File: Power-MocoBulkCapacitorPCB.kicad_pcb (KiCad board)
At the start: 2 copper layers, 120.5 x 44 mm, 142 parts, among them J1 Conn_01x02

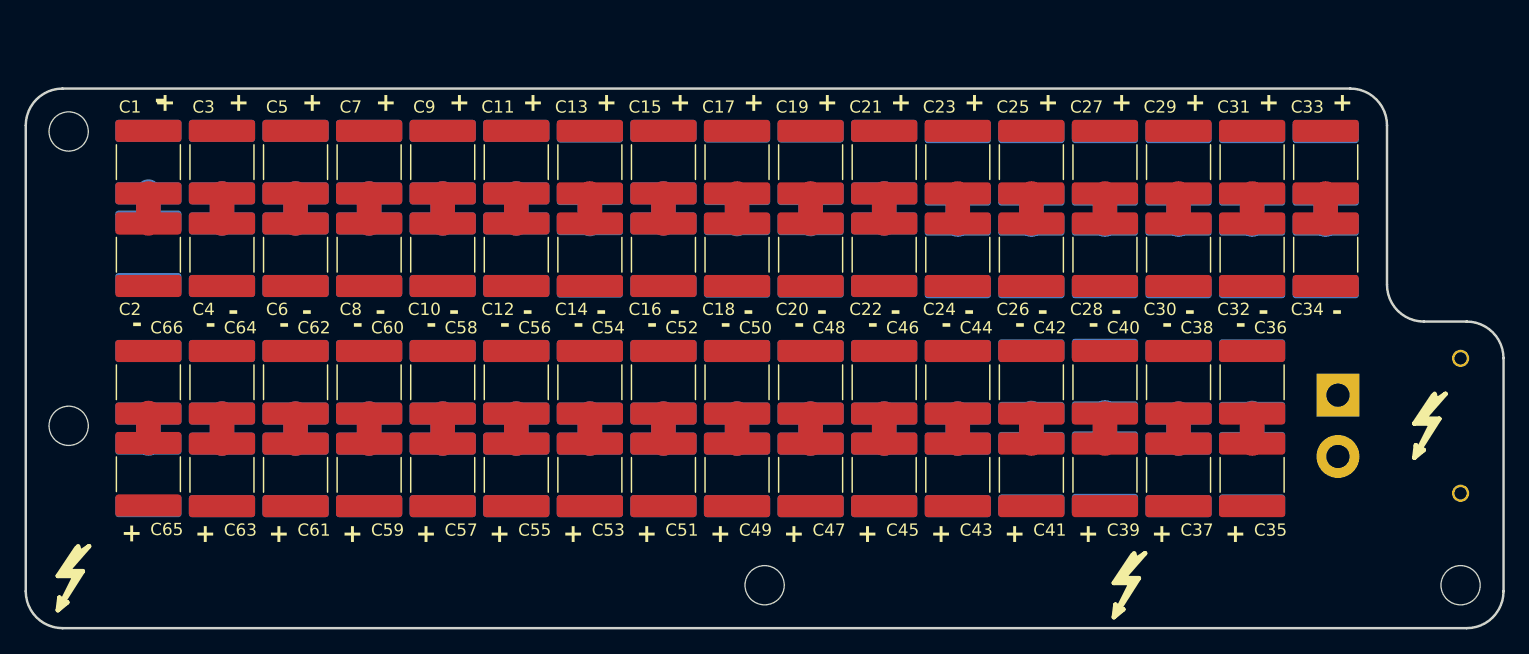
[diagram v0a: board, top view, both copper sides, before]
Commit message: holes
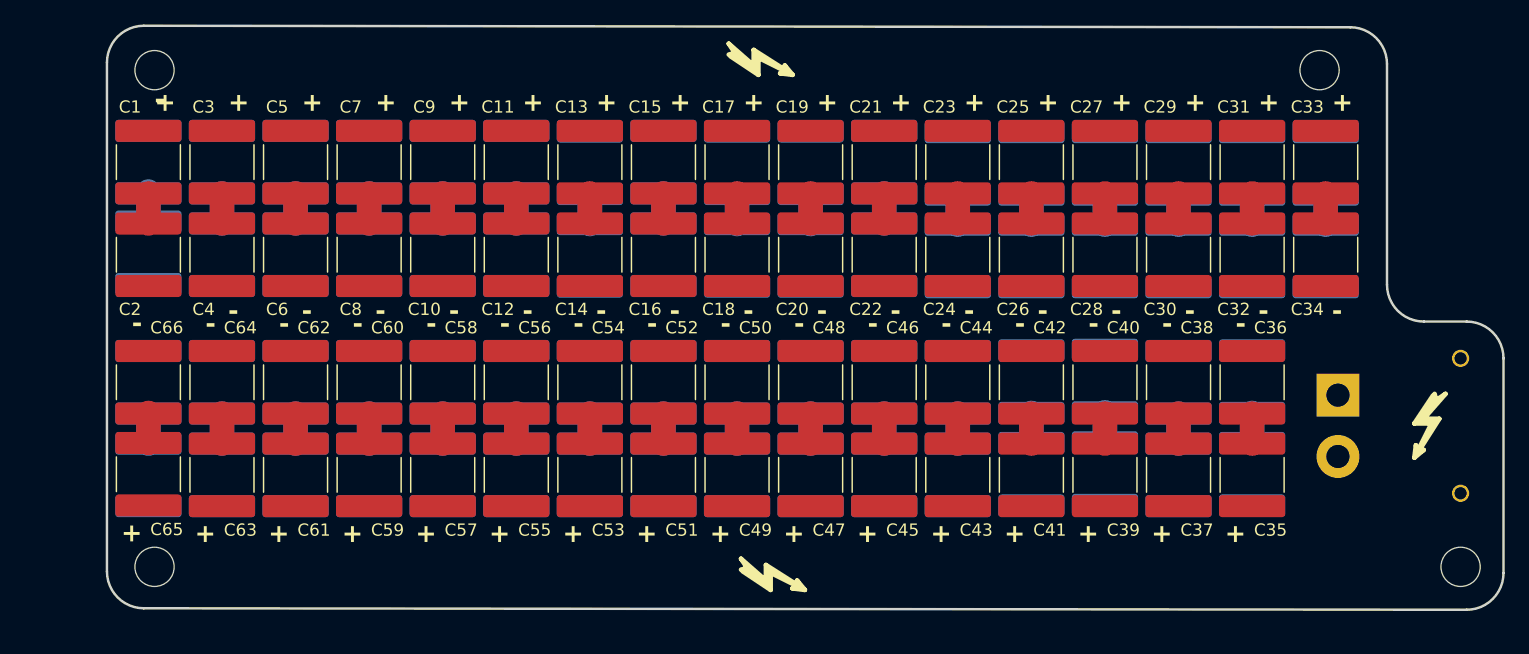
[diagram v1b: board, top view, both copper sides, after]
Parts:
- added REF**: Symbol_HighVoltage_Small, UTSVT_Special:Symbol_HighVoltage_Small, B.Cu at (209.9, 71.6)
- moved REF** 71.2 mm to (155.0, 42.0), turned to 90 degrees
- moved REF** 69.9 mm to (154.4, 41.1), turned to -90 degrees
- moved REF** 61.7 mm to (200.0, 42.0)
- moved REF** 28.9 mm to (156.6, 83.1), turned to -90 degrees
- moved REF** 27.6 mm to (156.0, 84.0), turned to 90 degrees
- moved REF** 13.5 mm to (105.0, 82.5)
- moved REF** 8.60 mm to (105.0, 42.0)
- moved REF** 1.50 mm to (211.5, 82.5)
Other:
- board size 120.5 x 44 mm -> 113.9 x 47.6 mm
